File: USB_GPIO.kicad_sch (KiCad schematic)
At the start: 22 parts, among them IC1 USBLC6-2SC6, IC5 TCA9534APWR, J1 PWM, Q1 SS8050-G, Q2 SS8050-G, SW1 Reset, SW2 Button, U1 USB-TYPE-C-018, U2 CP2102N-A02-GQFN28

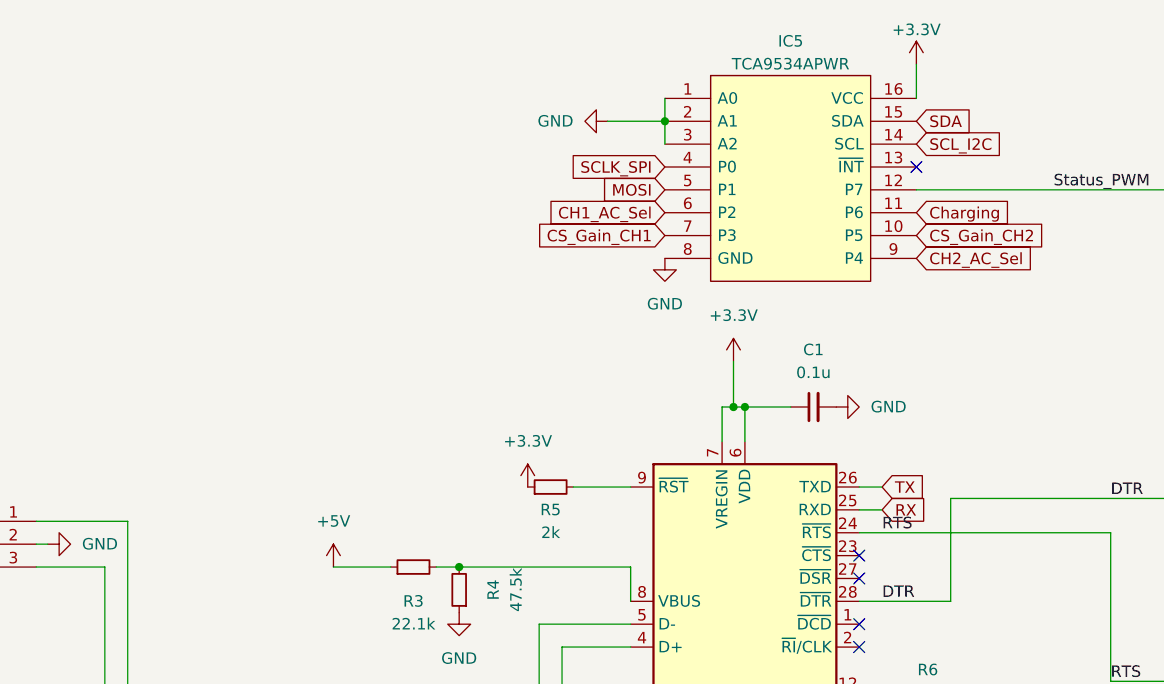
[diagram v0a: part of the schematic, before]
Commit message: last changes
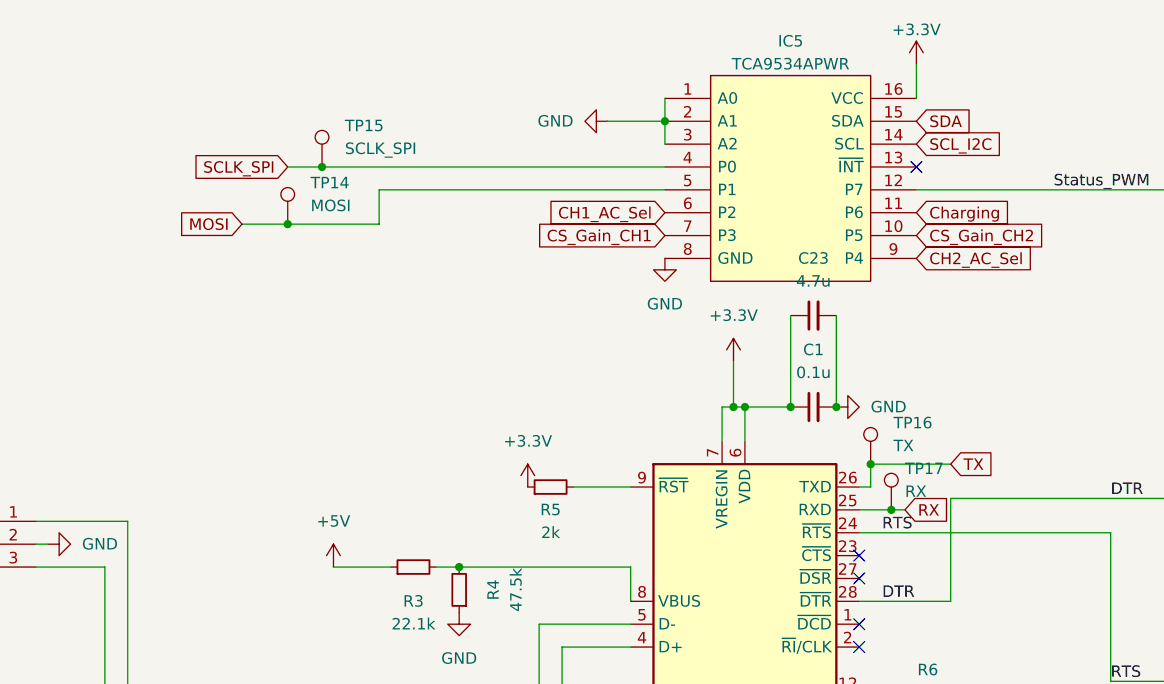
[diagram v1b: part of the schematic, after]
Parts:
- added C23: 4.7u, Capacitor_SMD:C_0603_1608Metric_Pad1.08x0.95mm_HandSolder, symbol Device:C_Small
- added TP14: MOSI, TestPoint:TestPoint_Keystone_5000-5004_Miniature, symbol Connector:TestPoint
- added TP15: SCLK_SPI, TestPoint:TestPoint_Keystone_5000-5004_Miniature, symbol Connector:TestPoint
- added TP16: TX, TestPoint:TestPoint_Keystone_5000-5004_Miniature, symbol Connector:TestPoint
- added TP17: RX, TestPoint:TestPoint_Keystone_5000-5004_Miniature, symbol Connector:TestPoint
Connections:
- net +3V3: now also C23.1
- net GND: now also C23.2
- net MOSI: now also TP14.1
- net RX: now also TP17.1
- net SCLK_SPI: now also TP15.1
- net TX: now also TP16.1
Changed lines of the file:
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@@
   (junction (at 73.66 85.09) (diameter 0) (color 0 0 0 0)
   )
+  (junction (at 142.24 64.77) (diameter 0) (color 0 0 0 0)
+  )
   (junction (at 241.3 60.96) (diameter 0) (color 0 0 0 0)
   )
+  (junction (at 209.3053 96.52) (diameter 0) (color 0 0 0 0)
+  )
   (junction (at 73.66 90.17) (diameter 0) (color 0 0 0 0)
   )
@@
   (junction (at 242.57 148.59) (diameter 0) (color 0 0 0 0)
   )
+  (junction (at 198.12 85.09) (diameter 0) (color 0 0 0 0)
+  )
   (junction (at 242.57 115.57) (diameter 0) (color 0 0 0 0)
   )
   (junction (at 243.84 95.25) (diameter 0) (color 0 0 0 0)
   )
+  (junction (at 146.05 58.42) (diameter 0) (color 0 0 0 0)
+  )
+  (junction (at 203.2 85.09) (diameter 0) (color 0 0 0 0)
+  )
   (junction (at 76.2 102.87) (diameter 0) (color 0 0 0 0)
   )
@@
   )
   (junction (at 191.77 85.09) (diameter 0) (color 0 0 0 0)
+  )
+  (junction (at 207.01 91.44) (diameter 0) (color 0 0 0 0)
   )
   (junction (at 248.92 129.54) (diameter 0) (color 0 0 0 0)
@@
   (no_connect (at 205.74 132.08))
   (no_connect (at 205.74 109.22))
-  (wire (pts (xy 205.74 93.98) (xy 208.28 93.98))
+  (wire (pts (xy 207.01 93.98) (xy 207.01 91.44))
     (stroke (width 0) (type default) (color 0 0 0 0))
   )
@@
     (stroke (width 0) (type default) (color 0 0 0 0))
   )
+  (wire (pts (xy 198.12 74.93) (xy 198.12 85.09))
+    (stroke (width 0) (type default) (color 0 0 0 0))
+  )
   (wire (pts (xy 242.57 158.75) (xy 248.92 158.75))
     (stroke (width 0) (type default) (color 0 0 0 0))
   )
+  (wire (pts (xy 203.2 74.93) (xy 203.2 85.09))
+    (stroke (width 0) (type default) (color 0 0 0 0))
+  )
   (wire (pts (xy 205.74 99.06) (xy 233.68 99.06))
     (stroke (width 0) (type default) (color 0 0 0 0))
   )
+  (wire (pts (xy 137.16 64.77) (xy 142.24 64.77))
+    (stroke (width 0) (type default) (color 0 0 0 0))
+  )
+  (wire (pts (xy 207.01 91.44) (xy 215.9 91.44))
+    (stroke (width 0) (type default) (color 0 0 0 0))
+  )
   (wire (pts (xy 172.72 124.46) (xy 172.72 111.76))
     (stroke (width 0) (type default) (color 0 0 0 0))
@@
     (stroke (width 0) (type default) (color 0 0 0 0))
   )
+  (wire (pts (xy 207.01 93.98) (xy 205.74 93.98))
+    (stroke (width 0) (type default) (color 0 0 0 0))
+  )
+  (wire (pts (xy 184.15 60.96) (xy 152.4 60.96))
+    (stroke (width 0) (type default) (color 0 0 0 0))
+  )
   (wire (pts (xy 85.09 118.11) (xy 85.09 123.19))
     (stroke (width 0) (type default) (color 0 0 0 0))
@@
     (stroke (width 0) (type default) (color 0 0 0 0))
   )
+  (wire (pts (xy 209.3053 96.52) (xy 210.82 96.52))
+    (stroke (width 0) (type default) (color 0 0 0 0))
+  )
   (wire (pts (xy 74.93 120.65) (xy 74.93 123.19))
     (stroke (width 0) (type default) (color 0 0 0 0))
@@
     (stroke (width 0) (type default) (color 0 0 0 0))
   )
+  (wire (pts (xy 152.4 60.96) (xy 152.4 64.77))
+    (stroke (width 0) (type default) (color 0 0 0 0))
+  )
   (wire (pts (xy 76.2 97.79) (xy 76.2 100.33))
     (stroke (width 0) (type default) (color 0 0 0 0))
@@
     (stroke (width 0) (type default) (color 0 0 0 0))
   )
-  (wire (pts (xy 205.74 96.52) (xy 208.28 96.52))
+  (wire (pts (xy 205.74 96.52) (xy 209.3053 96.52))
     (stroke (width 0) (type default) (color 0 0 0 0))
   )
@@
     (stroke (width 0) (type default) (color 0 0 0 0))
   )
+  (wire (pts (xy 146.05 58.42) (xy 184.15 58.42))
+    (stroke (width 0) (type default) (color 0 0 0 0))
+  )
   (wire (pts (xy 38.1 128.27) (xy 40.64 128.27))
     (stroke (width 0) (type default) (color 0 0 0 0))
@@
     (stroke (width 0) (type default) (color 0 0 0 0))
   )
+  (wire (pts (xy 142.24 58.42) (xy 146.05 58.42))
+    (stroke (width 0) (type default) (color 0 0 0 0))
+  )
   (wire (pts (xy 242.57 139.7) (xy 248.92 139.7))
+    (stroke (width 0) (type default) (color 0 0 0 0))
+  )
+  (wire (pts (xy 152.4 64.77) (xy 142.24 64.77))
     (stroke (width 0) (type default) (color 0 0 0 0))
   )
@@
     )
   )
-  (global_label "SCLK_SPI" (shape input) (at 184.15 58.42 180) (fields_autoplaced)
+  (global_label "SCLK_SPI" (shape input) (at 142.24 58.42 180) (fields_autoplaced)
     (effects (font (size 1.27 1.27)) (justify right))
-    (property "Intersheet References" "${INTERSHEET_REFS}" (id 0) (at 172.9074 58.3406 0)
+    (property "Intersheet References" "${INTERSHEET_REFS}" (id 0) (at 130.9974 58.3406 0)
       (effects (font (size 1.27 1.27)) (justify right) hide)
     )
   )
-  (global_label "MOSI" (shape input) (at 184.15 60.96 180) (fields_autoplaced)
+  (global_label "MOSI" (shape input) (at 137.16 64.77 180) (fields_autoplaced)
     (effects (font (size 1.27 1.27)) (justify right))
-    (property "Intersheet References" "${INTERSHEET_REFS}" (id 0) (at 177.1407 60.8806 0)
+    (property "Intersheet References" "${INTERSHEET_REFS}" (id 0) (at 130.1507 64.6906 0)
       (effects (font (size 1.27 1.27)) (justify right) hide)
     )
@@
     )
   )
-  (global_label "TX" (shape input) (at 208.28 93.98 0) (fields_autoplaced)
+  (global_label "TX" (shape input) (at 215.9 91.44 0) (fields_autoplaced)
     (effects (font (size 1.27 1.27)) (justify left))
-    (property "Intersheet References" "${INTERSHEET_REFS}" (id 0) (at 212.8702 93.9006 0)
-      (effects (font (size 1.27 1.27)) (justify left) hide)
-    )
-  )
-  (global_label "RX" (shape input) (at 208.28 96.52 0) (fields_autoplaced)
+    (property "Intersheet References" "${INTERSHEET_REFS}" (id 0) (at 220.4902 91.3606 0)
+      (effects (font (size 1.27 1.27)) (justify left) hide)
+    )
+  )
+  (global_label "RX" (shape input) (at 210.82 96.52 0) (fields_autoplaced)
     (effects (font (size 1.27 1.27)) (justify left))
-    (property "Intersheet References" "${INTERSHEET_REFS}" (id 0) (at 213.1726 96.4406 0)
+    (property "Intersheet References" "${INTERSHEET_REFS}" (id 0) (at 215.7126 96.4406 0)
       (effects (font (size 1.27 1.27)) (justify left) hide)
     )
@@
     (pin "5")
     (pin "6")
+  )
+  (symbol (lib_id "Device:C_Small") (at 200.66 74.93 90) (unit 1)
+    (in_bom yes) (on_board yes) (fields_autoplaced)
+    (property "Reference" "C23" (id 0) (at 200.6663 68.58 90))
+    (property "Value" "4.7u" (id 1) (at 200.6663 71.12 90))
+    (property "Footprint" "Capacitor_SMD:C_0603_1608Metric_Pad1.08x0.95mm_HandSolder" (id 2) (at 200.66 74.93 0)
+      (effects (font (size 1.27 1.27)) hide)
+    )
+    (property "Datasheet" "~" (id 3) (at 200.66 74.93 0)
+      (effects (font (size 1.27 1.27)) hide)
+    )
+    (pin "1")
+    (pin "2")
   )
   (symbol (lib_id "Device:C_Small") (at 248.92 153.67 0) (unit 1)
@@
     (pin "2")
   )
+  (symbol (lib_id "Connector:TestPoint") (at 207.01 91.44 0) (unit 1)
+    (in_bom yes) (on_board yes) (fields_autoplaced)
+    (property "Reference" "TP16" (id 0) (at 209.55 86.8679 0)
+      (effects (font (size 1.27 1.27)) (justify left))
+    )
+    (property "Value" "TX" (id 1) (at 209.55 89.4079 0)
+      (effects (font (size 1.27 1.27)) (justify left))
+    )
+    (property "Footprint" "TestPoint:TestPoint_Keystone_5000-5004_Miniature" (id 2) (at 212.09 91.44 0)
+      (effects (font (size 1.27 1.27)) hide)
+    )
+    (property "Datasheet" "~" (id 3) (at 212.09 91.44 0)
+      (effects (font (size 1.27 1.27)) hide)
+    )
+    (pin "1")
+  )
   (symbol (lib_id "Device:R_Small") (at 171.45 93.98 90) (unit 1)
     (in_bom yes) (on_board yes)
@@
     )
     (property "Datasheet" "" (id 3) (at 85.09 130.81 0)
+      (effects (font (size 1.27 1.27)) hide)
+    )
+    (pin "1")
+  )
+  (symbol (lib_id "Connector:TestPoint") (at 209.3053 96.52 0) (unit 1)
+    (in_bom yes) (on_board yes) (fields_autoplaced)
+    (property "Reference" "TP17" (id 0) (at 210.82 91.9479 0)
+      (effects (font (size 1.27 1.27)) (justify left))
+    )
+    (property "Value" "RX" (id 1) (at 210.82 94.4879 0)
+      (effects (font (size 1.27 1.27)) (justify left))
+    )
+    (property "Footprint" "TestPoint:TestPoint_Keystone_5000-5004_Miniature" (id 2) (at 214.3853 96.52 0)
+      (effects (font (size 1.27 1.27)) hide)
+    )
+    (property "Datasheet" "~" (id 3) (at 214.3853 96.52 0)
       (effects (font (size 1.27 1.27)) hide)
     )
@@
     (pin "2")
   )
+  (symbol (lib_id "Connector:TestPoint") (at 142.24 64.77 0) (unit 1)
+    (in_bom yes) (on_board yes) (fields_autoplaced)
+    (property "Reference" "TP14" (id 0) (at 144.78 60.1979 0)
+      (effects (font (size 1.27 1.27)) (justify left))
+    )
+    (property "Value" "MOSI" (id 1) (at 144.78 62.7379 0)
+      (effects (font (size 1.27 1.27)) (justify left))
+    )
+    (property "Footprint" "TestPoint:TestPoint_Keystone_5000-5004_Miniature" (id 2) (at 147.32 64.77 0)
+      (effects (font (size 1.27 1.27)) hide)
+    )
+    (property "Datasheet" "~" (id 3) (at 147.32 64.77 0)
+      (effects (font (size 1.27 1.27)) hide)
+    )
+    (pin "1")
+  )
+  (symbol (lib_id "Connector:TestPoint") (at 146.05 58.42 0) (unit 1)
+    (in_bom yes) (on_board yes) (fields_autoplaced)
+    (property "Reference" "TP15" (id 0) (at 148.59 53.8479 0)
+      (effects (font (size 1.27 1.27)) (justify left))
+    )
+    (property "Value" "SCLK_SPI" (id 1) (at 148.59 56.3879 0)
+      (effects (font (size 1.27 1.27)) (justify left))
+    )
+    (property "Footprint" "TestPoint:TestPoint_Keystone_5000-5004_Miniature" (id 2) (at 151.13 58.42 0)
+      (effects (font (size 1.27 1.27)) hide)
+    )
+    (property "Datasheet" "~" (id 3) (at 151.13 58.42 0)
+      (effects (font (size 1.27 1.27)) hide)
+    )
+    (pin "1")
+  )
   (symbol (lib_id "power:+3.3V") (at 168.91 93.98 0) (unit 1)
